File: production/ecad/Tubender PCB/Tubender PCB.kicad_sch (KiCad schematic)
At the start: 0 parts

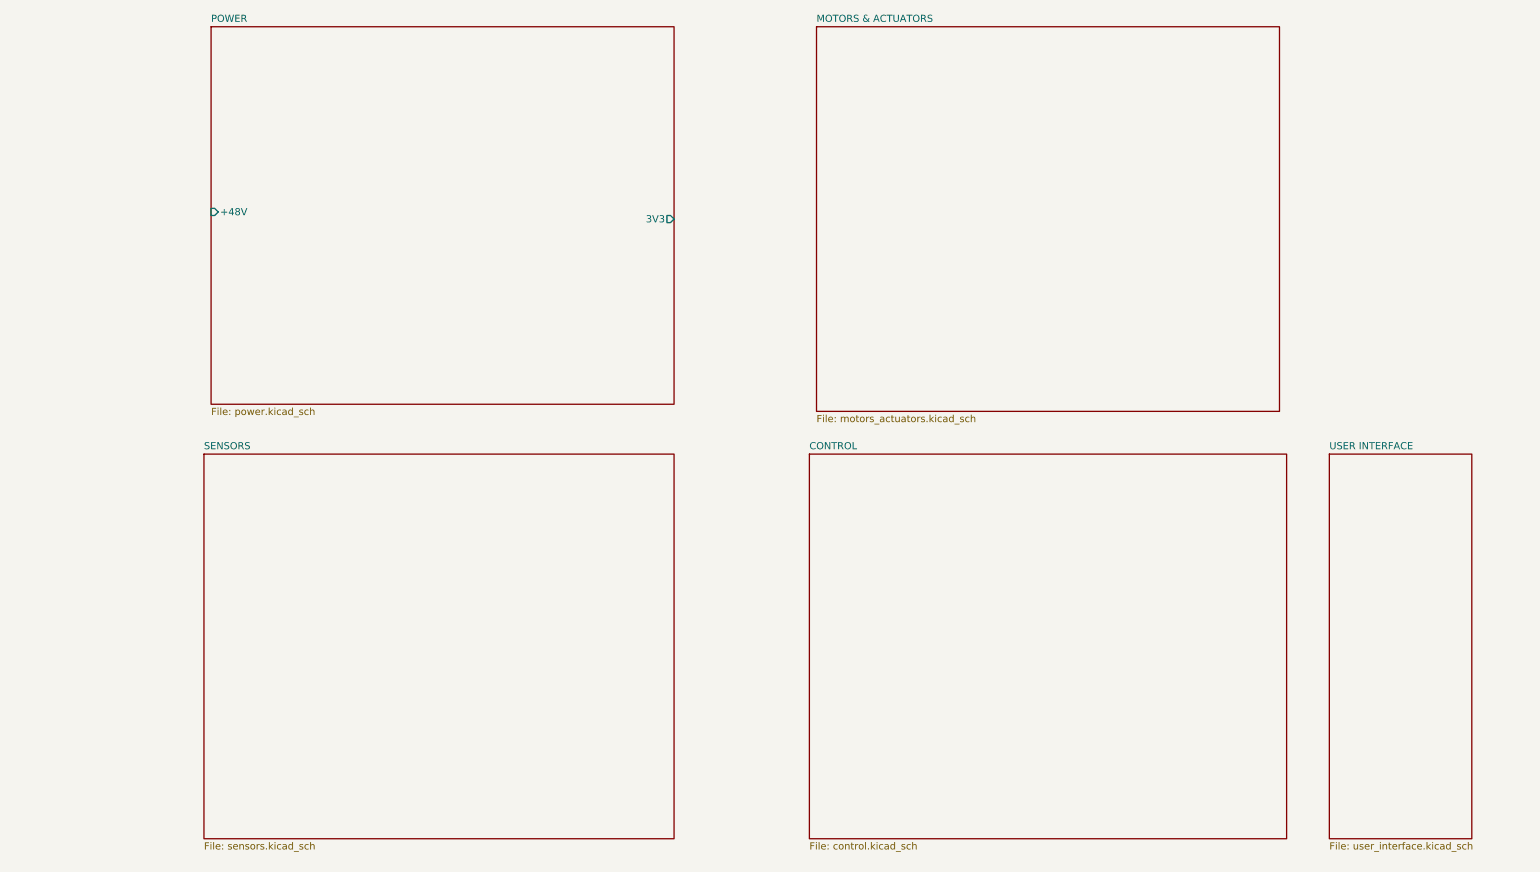
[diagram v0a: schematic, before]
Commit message: Fixed Button Connectors
All done! Enjoy :)
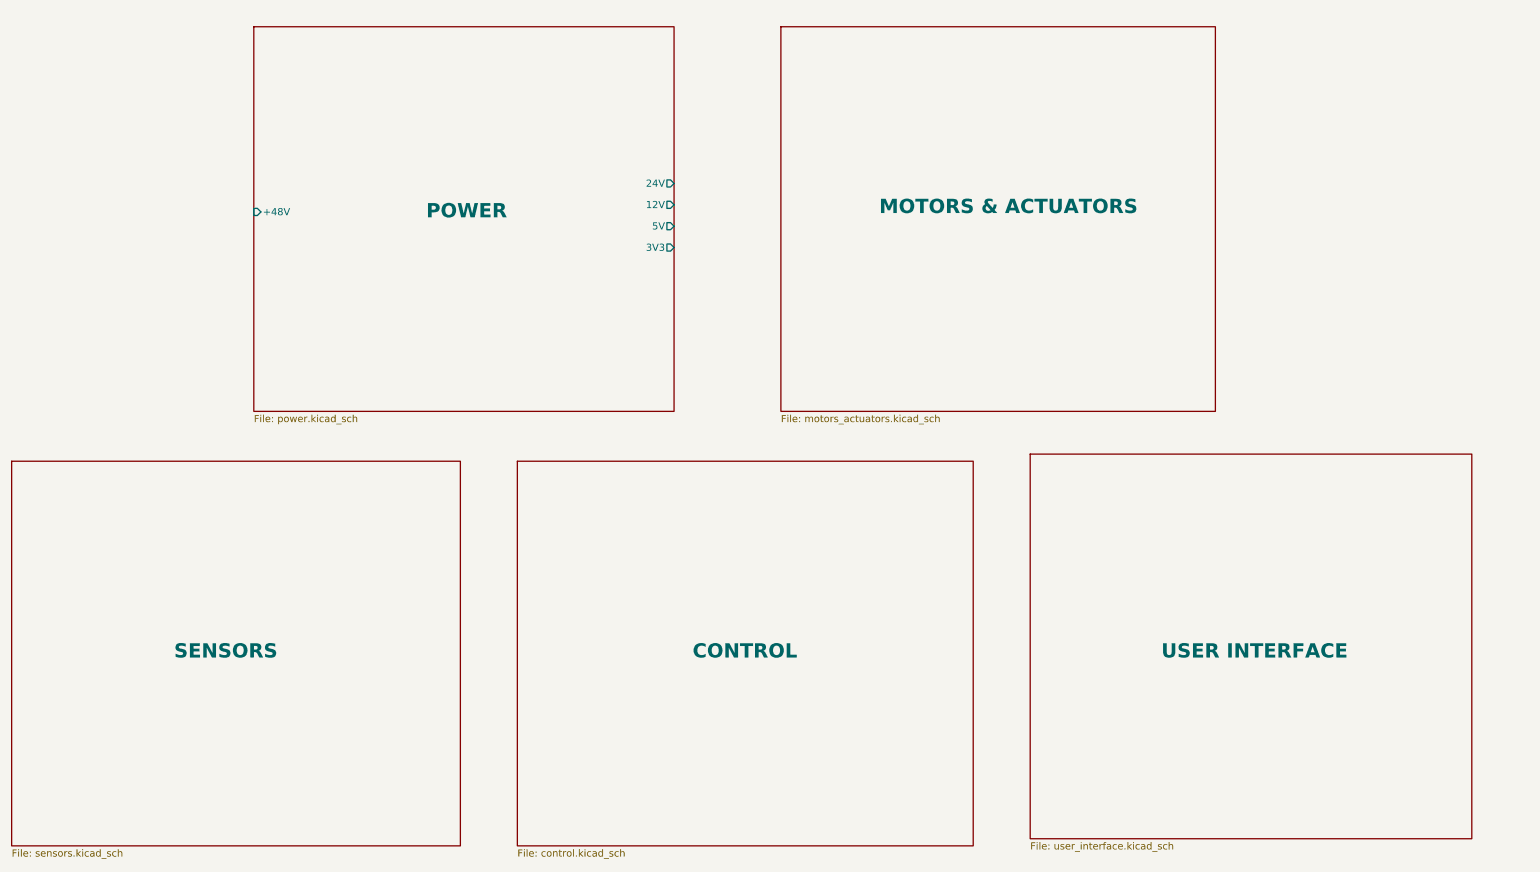
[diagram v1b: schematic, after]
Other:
- sheet POWER ports: added 12V, 24V, 5V; removed none
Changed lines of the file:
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@@
 	)
 	(sheet
-		(at 160.02 17.78)
-		(size 82.55 68.58)
-		(fields_autoplaced yes)
+		(at 153.67 17.78)
+		(size 77.47 68.58)
 		(stroke
 			(width 0.1524)
@@
 		)
 		(property "Sheetname" "MOTORS & ACTUATORS"
-			(at 160.02 17.0684 0)
-			(effects
-				(font
-					(size 1.27 1.27)
+			(at 171.196 51.308 0)
+			(effects
+				(font
+					(size 2.54 2.54)
+					(thickness 0.508)
+					(bold yes)
 				)
 				(justify left bottom)
@@
 		)
 		(property "Sheetfile" "motors_actuators.kicad_sch"
-			(at 160.02 86.9446 0)
+			(at 153.67 86.9446 0)
 			(effects
 				(font
@@
 	)
 	(sheet
-		(at 52.07 17.78)
-		(size 82.55 67.31)
-		(fields_autoplaced yes)
+		(at 59.69 17.78)
+		(size 74.93 68.58)
 		(stroke
 			(width 0.1524)
@@
 		)
 		(property "Sheetname" "POWER"
-			(at 52.07 17.0684 0)
-			(effects
-				(font
-					(size 1.27 1.27)
+			(at 90.424 52.07 0)
+			(effects
+				(font
+					(size 2.54 2.54)
+					(thickness 0.508)
+					(bold yes)
 				)
 				(justify left bottom)
@@
 		)
 		(property "Sheetfile" "power.kicad_sch"
-			(at 52.07 85.6746 0)
+			(at 59.69 86.9446 0)
 			(effects
 				(font
@@
 		)
 		(pin "3V3" output
-			(at 134.62 52.07 0)
+			(at 134.62 57.15 0)
 			(effects
 				(font
@@
 		)
 		(pin "+48V" input
-			(at 52.07 50.8 180)
+			(at 59.69 50.8 180)
 			(effects
 				(font
@@
 			)
 		)
+		(pin "12V" output
+			(at 134.62 49.53 0)
+			(effects
+				(font
+					(size 1.27 1.27)
+				)
+				(justify right)
+			)
+		)
+		(pin "5V" output
+			(at 134.62 53.34 0)
+			(effects
+				(font
+					(size 1.27 1.27)
+				)
+				(justify right)
+			)
+		)
+		(pin "24V" output
+			(at 134.62 45.72 0)
+			(effects
+				(font
+					(size 1.27 1.27)
+				)
+				(justify right)
+			)
+		)
 		(instances
 			(project "Tubender PCB"
@@
 	)
 	(sheet
-		(at 158.75 93.98)
-		(size 85.09 68.58)
-		(fields_autoplaced yes)
+		(at 106.68 95.25)
+		(size 81.28 68.58)
 		(stroke
 			(width 0.1524)
@@
 		)
 		(property "Sheetname" "CONTROL"
-			(at 158.75 93.2684 0)
-			(effects
-				(font
-					(size 1.27 1.27)
+			(at 137.922 130.556 0)
+			(effects
+				(font
+					(size 2.54 2.54)
+					(thickness 0.508)
+					(bold yes)
 				)
 				(justify left bottom)
@@
 		)
 		(property "Sheetfile" "control.kicad_sch"
-			(at 158.75 163.1446 0)
+			(at 106.68 164.4146 0)
 			(effects
 				(font
@@
 	)
 	(sheet
-		(at 50.8 93.98)
-		(size 83.82 68.58)
-		(fields_autoplaced yes)
+		(at 16.51 95.25)
+		(size 80.01 68.58)
 		(stroke
 			(width 0.1524)
@@
 		)
 		(property "Sheetname" "SENSORS"
-			(at 50.8 93.2684 0)
-			(effects
-				(font
-					(size 1.27 1.27)
+			(at 45.466 130.556 0)
+			(effects
+				(font
+					(size 2.54 2.54)
+					(thickness 0.508)
+					(bold yes)
 				)
 				(justify left bottom)
@@
 		)
 		(property "Sheetfile" "sensors.kicad_sch"
-			(at 50.8 163.1446 0)
+			(at 16.51 164.4146 0)
 			(effects
 				(font
@@
 	)
 	(sheet
-		(at 251.46 93.98)
-		(size 25.4 68.58)
-		(fields_autoplaced yes)
+		(at 198.12 93.98)
+		(size 78.74 68.58)
 		(stroke
 			(width 0.1524)
@@
 		)
 		(property "Sheetname" "USER INTERFACE"
-			(at 251.46 93.2684 0)
-			(effects
-				(font
-					(size 1.27 1.27)
+			(at 221.488 130.556 0)
+			(effects
+				(font
+					(size 2.54 2.54)
+					(thickness 0.508)
+					(bold yes)
 				)
 				(justify left bottom)
@@
 		)
 		(property "Sheetfile" "user_interface.kicad_sch"
-			(at 251.46 163.1446 0)
-			(effects
-				(font
+			(at 198.12 163.1446 0)
+			(effects
+				(font
